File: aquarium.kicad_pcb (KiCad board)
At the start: 2 copper layers, 190.8 x 47 mm, 70 parts, among them T1 E16, U1 MOC3063, U2 PC817A

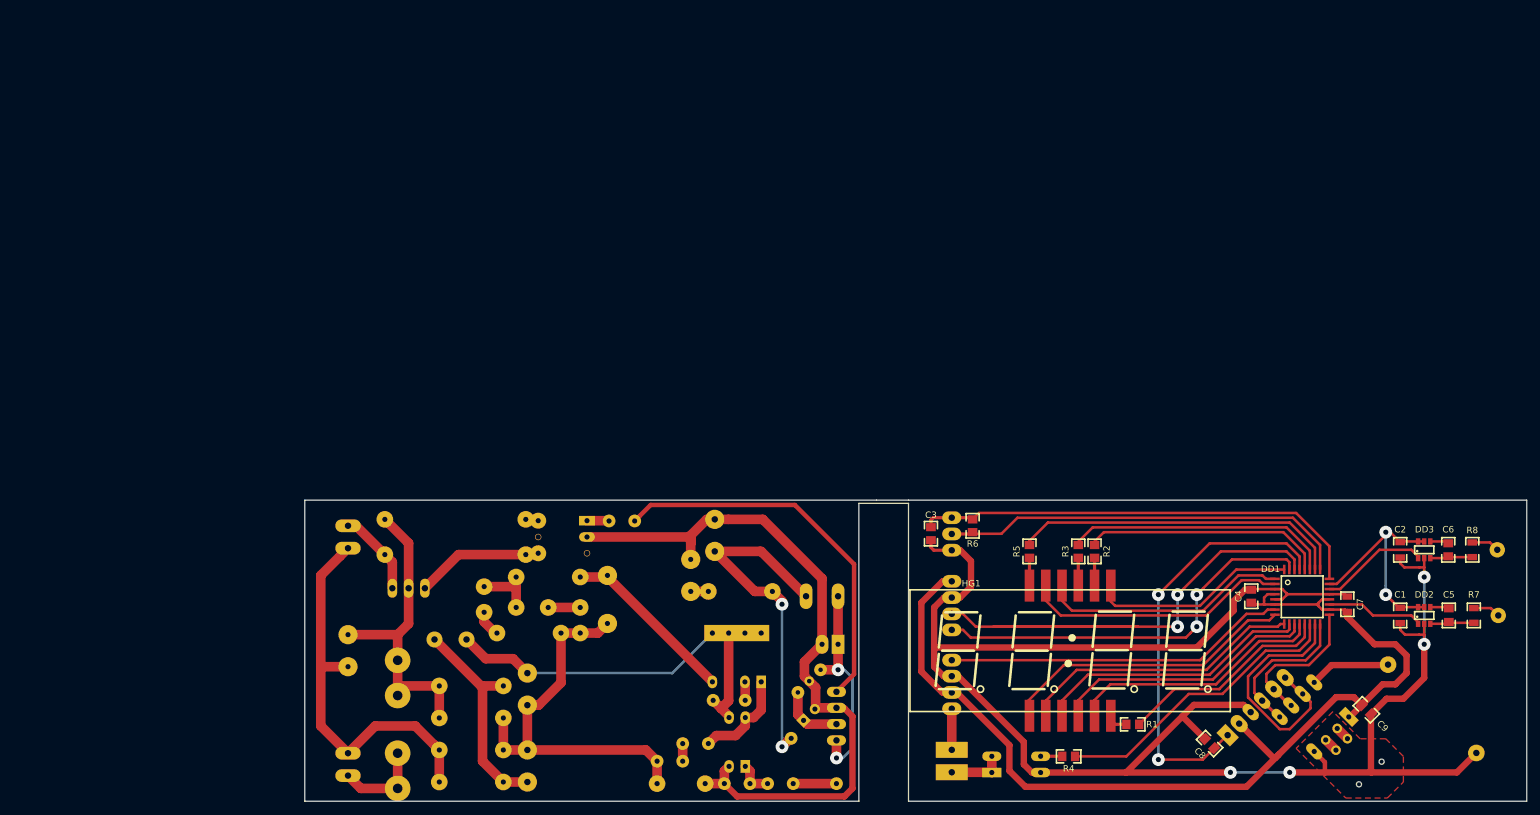
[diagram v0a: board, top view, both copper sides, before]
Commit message: Finished working on PCB.
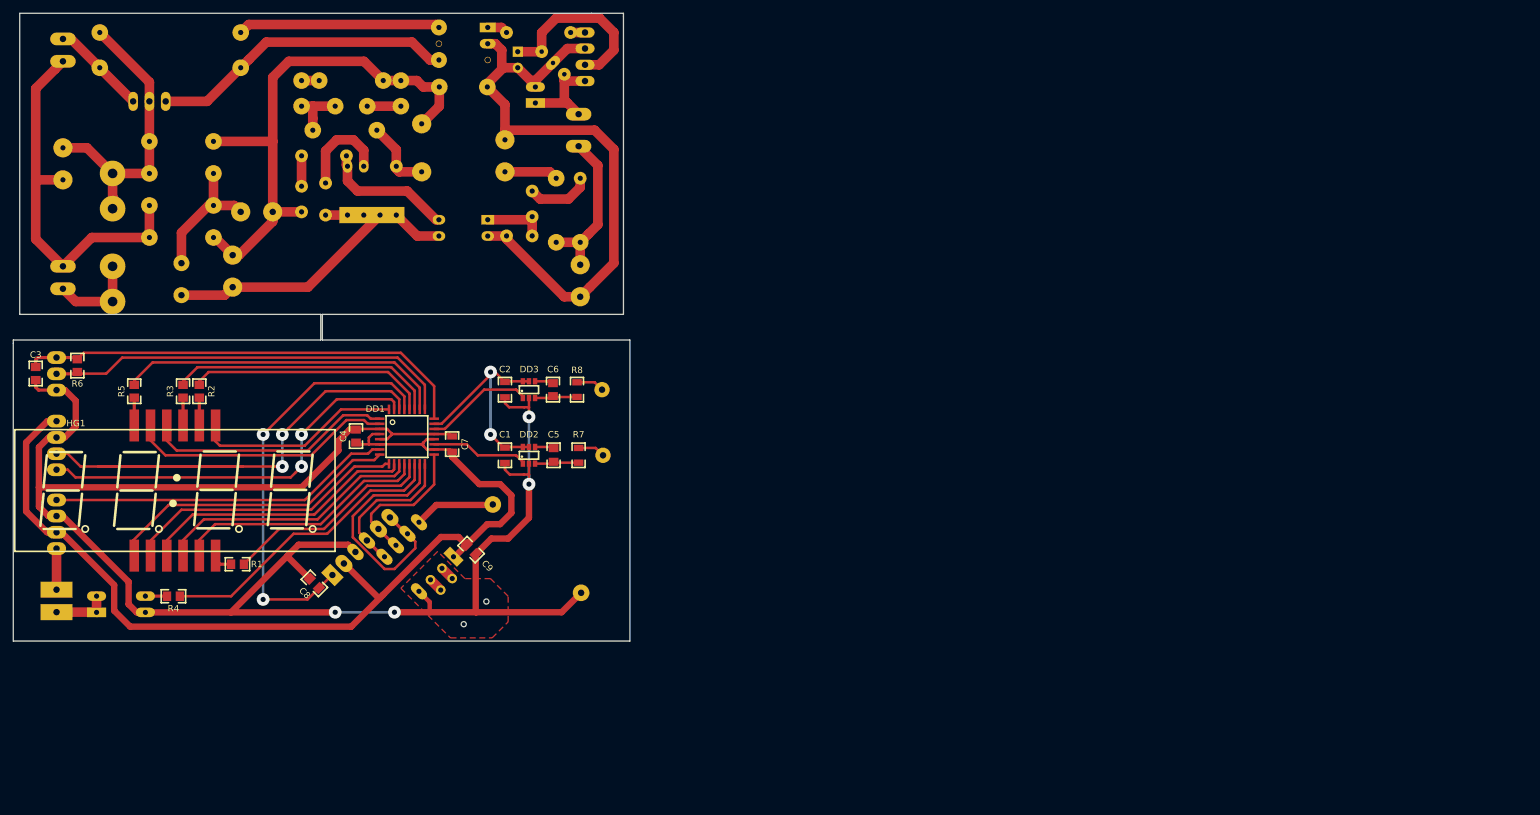
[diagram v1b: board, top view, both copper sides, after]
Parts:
- added G***: LOGO, aquarium:oshw-logo, B.Cu at (28.8, 75.2)
- added REF**: Symbol_HighVoltage_Type2_CopperTop_VerySmall, Symbols:Symbol_HighVoltage_Type2_CopperTop_VerySmall, B.Cu at (55.8, 7.50)
- R11: footprint Резисторы:RV_0.25 -> Резисторы:RH_0.25
- moved C1 142.0 mm to (80.8, 72.0)
- moved C2 142.0 mm to (80.8, 61.8)
- moved C3 142.0 mm to (7.50, 59.2)
- moved C4 142.0 mm to (57.5, 69.0)
- moved C5 142.0 mm to (88.3, 72.0)
- moved C6 142.0 mm to (88.2, 61.8)
- moved C7 142.0 mm to (72.5, 70.2)
- moved C8 142.0 mm to (51.0, 92.0)
- moved C9 142.0 mm to (75.5, 86.7)
- moved DD1 142.0 mm to (65.4, 69.1)
- moved DD2 142.0 mm to (84.5, 72.0)
- moved DD3 142.0 mm to (84.5, 61.8)
- moved DD4 142.0 mm to (67.3, 87.8)
- moved DD5 142.0 mm to (10.8, 59.3)
- moved GB1 142.0 mm to (85.7, 86.6)
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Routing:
- net Net-(R11-Pad2): track 60.2 -> 2.25 mm
- net Net-(C15-Pad1): track 55.6 -> 24.6 mm, vias 2 -> 0
- net Net-(R9-Pad1): track 2.03 -> 31.6 mm
- net Net-(R10-Pad1): track 20.0 -> 47.6 mm
- net Net-(C10-Pad1): track 62.5 -> 84.4 mm
- net Net-(C11-Pad2): track 66.7 -> 47.6 mm
- net +12B: track 40.4 -> 21.8 mm, vias 2 -> 0
- net +5B: track 169.0 -> 186.9 mm
- net Net-(DA1-Pad4): track 27.4 -> 11.5 mm
- net GND: track 395.8 -> 381.3 mm
- net Net-(C10-Pad2): track 33.8 -> 21.2 mm
- net Net-(C12-Pad1): track 2.90 -> 14.9 mm
- net Net-(T1-Pad3): track 2.75 -> 8.41 mm
- net Net-(DA1-Pad1): track 15.6 -> 20.8 mm
- net Net-(R16-Pad2): track 5.74 -> 10.1 mm
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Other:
- board size 190.8 x 47 mm -> 96.2 x 98 mm
- board text added: "SENSOR 1"
- board text added: "SENSOR 2"
